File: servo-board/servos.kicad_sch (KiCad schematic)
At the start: 19 parts, among them M1 Motor_Servo, M2 Motor_Servo, M3 Motor_Servo, M4 Motor_Servo, M5 Motor_Servo, M6 Motor_Servo, M7 Motor_Servo, M8 Motor_Servo, P1 SolderBridge_GND, P2 SolderBridge_GND, P3 SolderBridge_GND, P4 SolderBridge_GND, P5 SolderBridge_GND, U3 ADUM1401CRWZ, U4 ADUM1401CRWZ, U5 LDO_MIC5206-5.0YM5-TR

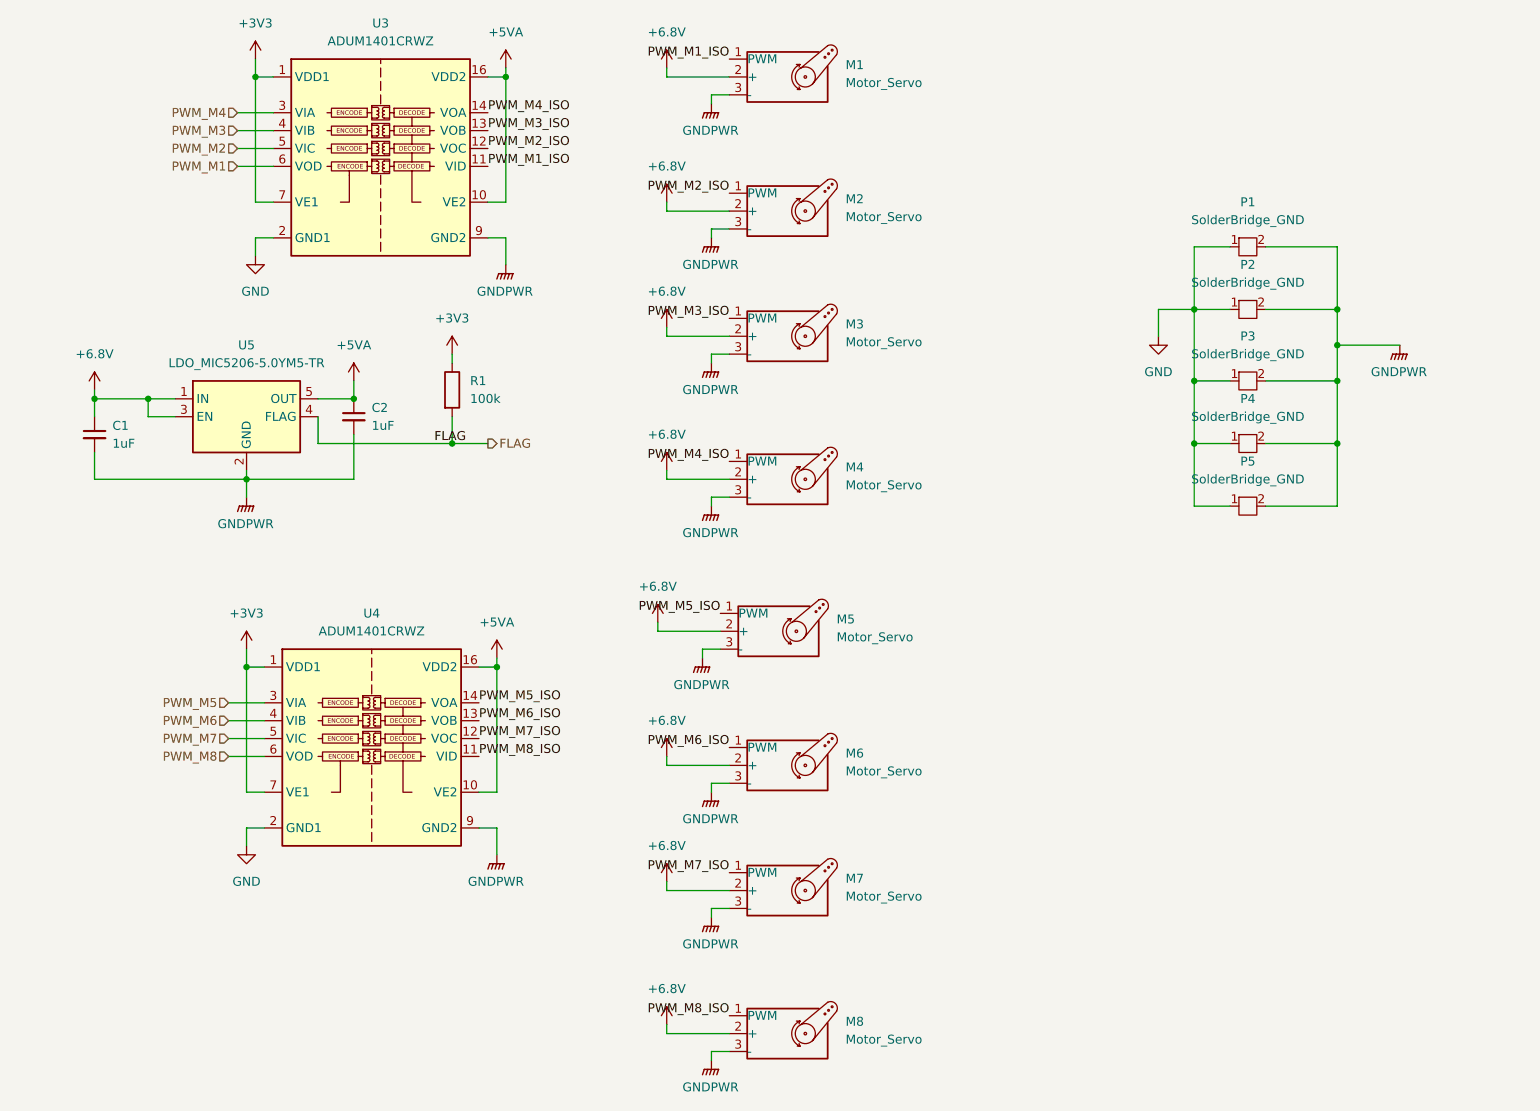
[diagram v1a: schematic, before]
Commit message: changes
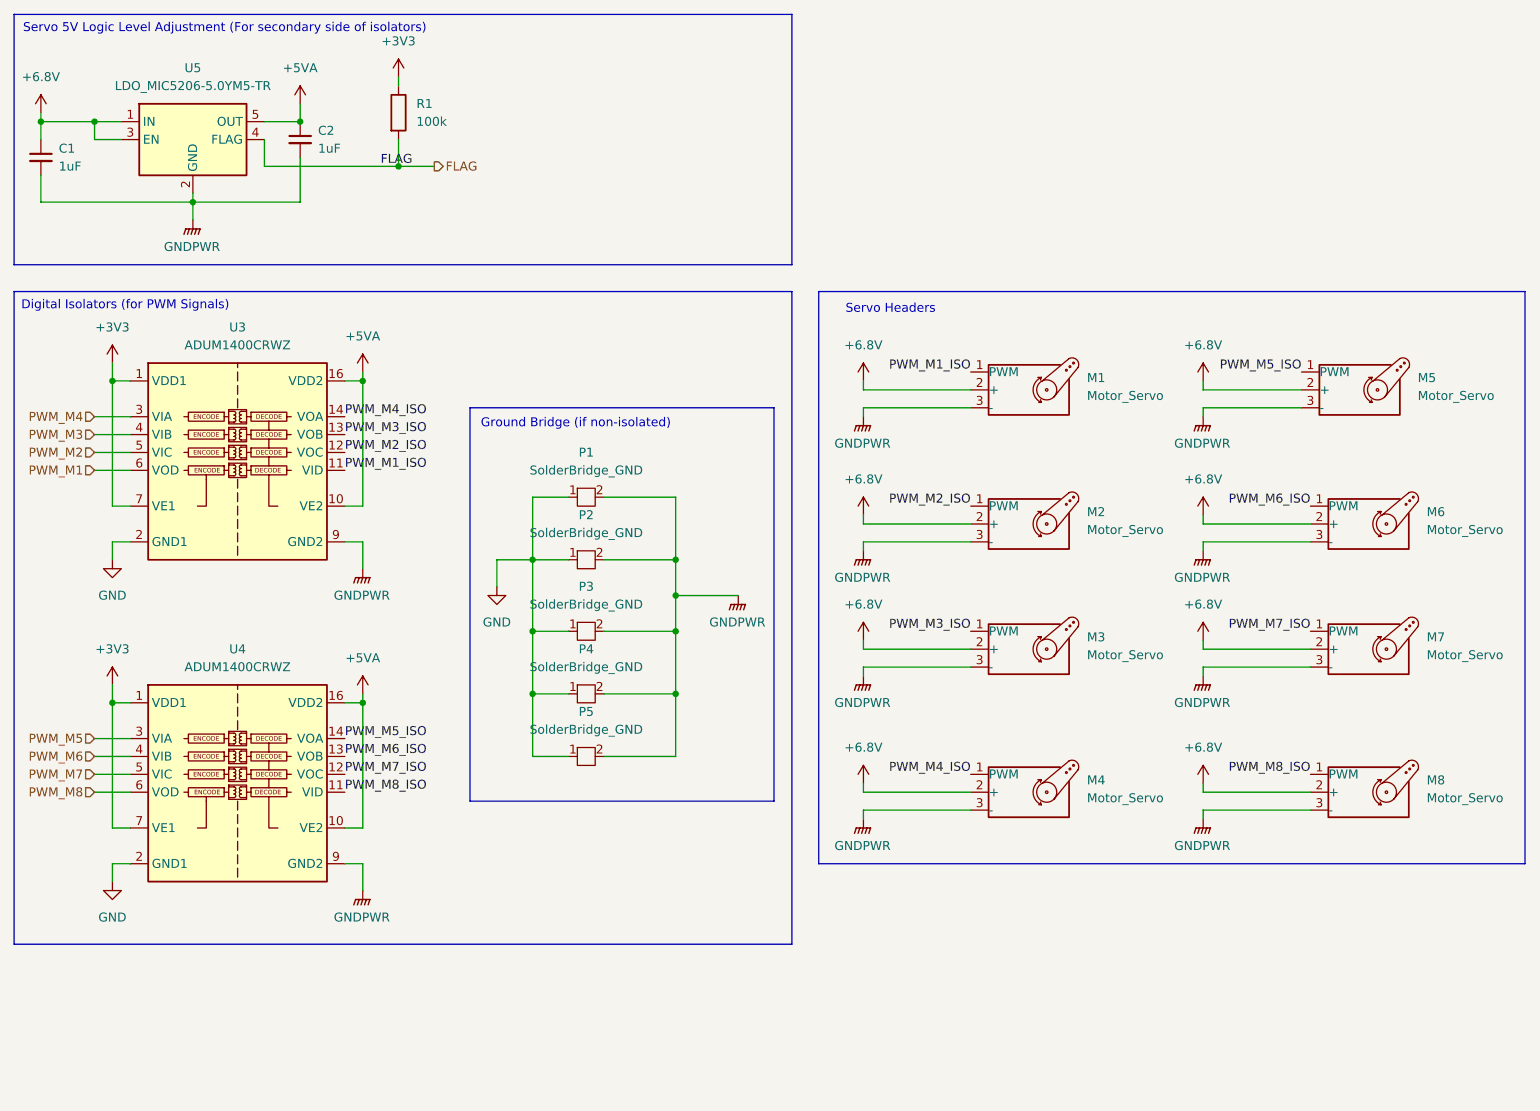
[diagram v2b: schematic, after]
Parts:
- U3, U4: value ADUM1401CRWZ -> ADUM1400CRWZ; symbol bio-robot:ADUM1401CRWZ -> bio-robot:ADUM1400CRWZ
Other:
- note added: "Digital Isolators (for PWM Signals)"
- note added: "Ground Bridge (if non-isolated)"
- note added: "Servo 5V Logic Level Adjustment (For secondary side of isolators)"
- note added: "Servo Headers"
- moved on the sheet: C1, C2, M1, M2, M3, M4, M5, M6, M7, M8, P1, P2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
